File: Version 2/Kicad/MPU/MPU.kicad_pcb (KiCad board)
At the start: 2 copper layers, 25.9 x 27.5 mm, 16 parts, among them U1 AMS1117-3.3, U2 MPU-6050

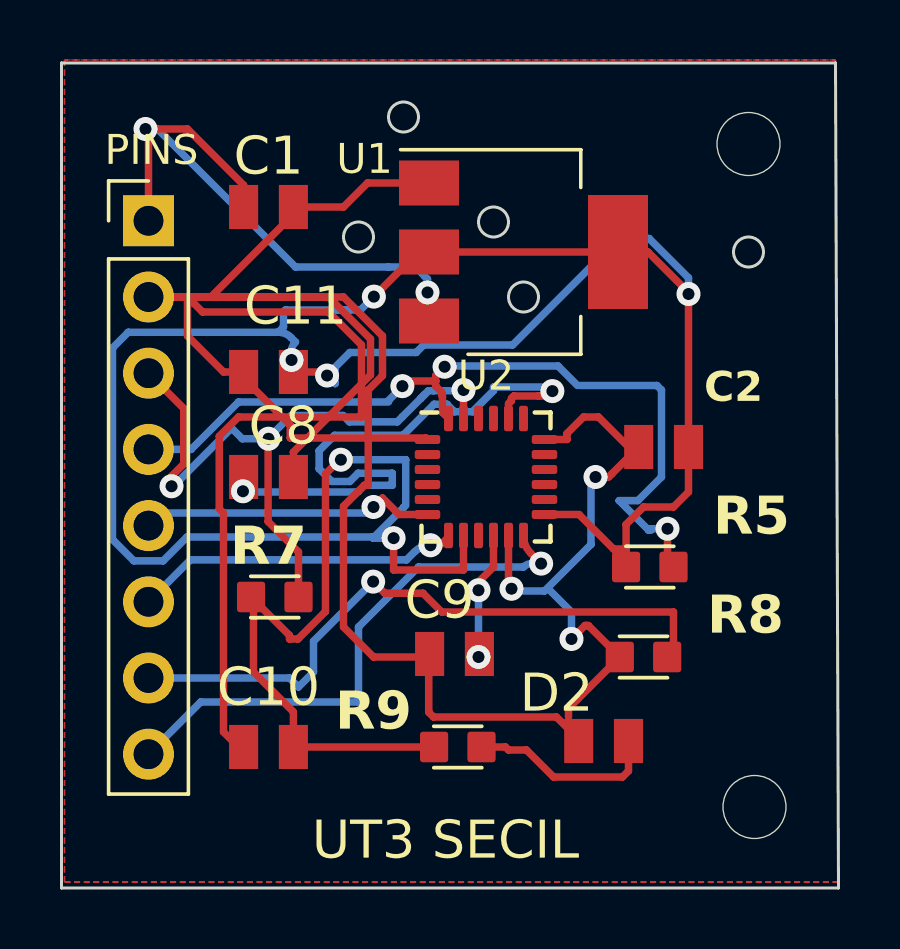
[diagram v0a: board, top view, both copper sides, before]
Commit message: Modified: rerouting the pcb
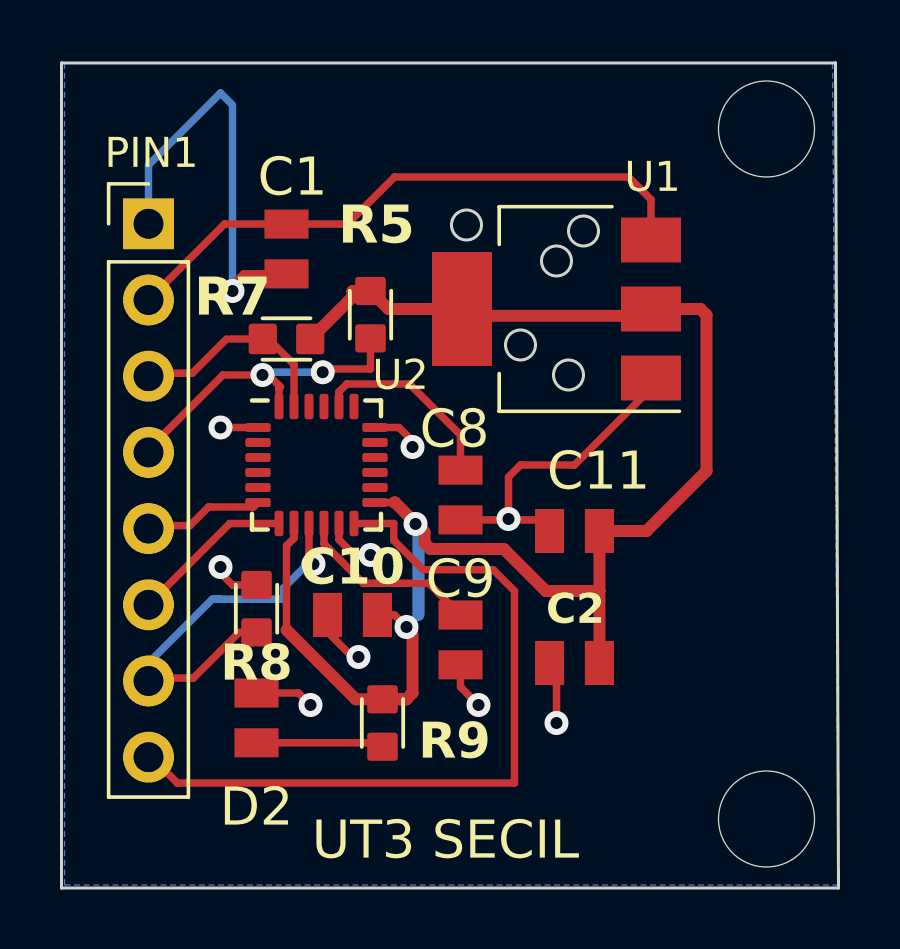
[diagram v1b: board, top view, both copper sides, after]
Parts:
- removed the REF** at (94.2, 72.0)
- removed the REF** at (94.0, 49.9)
- added REF**: MountingHole_3.2mm_M3, MountingHole:MountingHole_3.2mm_M3, F.Cu at (94.6, 49.4)
- added REF**: MountingHole_3.2mm_M3, MountingHole:MountingHole_3.2mm_M3, F.Cu at (94.6, 72.4)
- moved R8 13.0 mm to (77.6, 65.4), turned to -90 degrees
- moved R5 12.5 mm to (81.4, 55.6), turned to -90 degrees
- moved D2 11.6 mm to (77.6, 69.0), turned to -90 degrees
- moved C11 11.5 mm to (88.2, 62.8)
- moved R7 8.61 mm to (78.6, 56.4), turned to 180 degrees
- moved C2 7.79 mm to (88.2, 67.2)
- moved C8 6.43 mm to (84.4, 61.6), turned to -90 degrees
- moved U2 5.66 mm to (79.6, 60.6)
- moved C10 5.22 mm to (80.8, 65.6)
- moved R9 2.63 mm to (81.8, 69.2), turned to -90 degrees
- moved U1 2.20 mm to (87.6, 55.4), turned to 180 degrees
- moved C1 1.52 mm to (78.6, 53.4), turned to 90 degrees
- moved C9 0.51 mm to (84.4, 66.4), turned to 90 degrees
- moved PIN1 0.10 mm to (74.0, 52.6)
- renumbered PINS to PIN1
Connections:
- PIN1 pad 1: VCC -> GND
- PIN1 pad 2: GND -> VCC
- PIN1 pad 7: Net-(PIN1-Pin_7) -> /AD0
- R8 pad 2: Net-(PIN1-Pin_7) -> /AD0
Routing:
- net GND: track 110.1 -> 38.9 mm, vias 3 -> 10
- net +3.3V: track 100.7 -> 53.6 mm, vias 6 -> 2
- net Net-(PIN1-Pin_7): track 21.7 -> 0.00 mm, vias 1 -> 0
- net /SDA: track 28.2 -> 11.0 mm, vias 3 -> 2
- net /SCL: track 22.8 -> 6.95 mm, vias 3 -> 0
- net Net-(U2-CPOUT): track 20.0 -> 6.52 mm, vias 2 -> 0
- net /AD0: track 0.00 -> 13.1 mm, vias 0 -> 1
- net /INT: track 18.3 -> 25.6 mm, vias 1 -> 0
- net /XDA: track 9.91 -> 3.97 mm, vias 1 -> 0
- net /XCL: track 11.0 -> 5.47 mm, vias 1 -> 0
- net Net-(D2-A): track 6.40 -> 4.25 mm
- net Net-(U2-REGOUT): track 4.71 -> 6.21 mm, vias 2 -> 0
- net VCC: track 20.8 -> 20.1 mm, vias 2 -> 0
- added copper zone on B.Cu, net GND
- removed copper zone on F.Cu, net +3.3V
- removed copper zone on F.Cu, net GND
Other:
- outline, holes or cut-outs redrawn
